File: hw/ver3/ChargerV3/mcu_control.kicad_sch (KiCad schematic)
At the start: 58 parts, among them J6 BMS_Serial, J7 Debug, J8 SWD Debug, J9 USB_B_Micro, Q12 BSS138, Q13 BSS138, Q14 BSS138, Q15 BSS84, Q16 BSS138, Q19 BSS138, Q30 BSS138, SW1 Boot, SW2 Reset, U12 W25Q32JVZP, U18 RP2040, U21 W25Q32JVZP, Y1 12MHz

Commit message: Nearly final charger schematic, updated with RS485 interconnect.
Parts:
- removed C24: 100nF, Capacitor_SMD:C_0603_1608Metric, symbol Device:C
- removed D19: Yellow LED, LED_SMD:LED_0805_2012Metric, symbol Device:LED
- removed J6: BMS_Serial, Connector_PinHeader_2.54mm:PinHeader_1x03_P2.54mm_Vertical, symbol Connector:Conn_01x03_Pin
- removed Q30: BSS138, Package_TO_SOT_SMD:SOT-23, symbol Transistor_FET:BSS138
- removed R115: 510, Resistor_SMD:R_0603_1608Metric, symbol Device:R_US
- removed R5, R97: 10k, Resistor_SMD:R_0603_1608Metric, symbol Device:R_US
- removed R58, R59: 100, Resistor_SMD:R_0603_1608Metric, symbol Device:R_US
- added J5: FanConnector, Connector_Molex:Molex_KK-254_AE-6410-04A_1x04_P2.54mm_Vertical, symbol Connector:Conn_01x04_Pin
- added R55, R56: 100, Resistor_SMD:R_0603_1608Metric, symbol Device:R_US
- added R57: 10k, Resistor_SMD:R_0603_1608Metric, symbol Device:R_US
- added R92: 1k, Resistor_SMD:R_0603_1608Metric, symbol Device:R_US
- J9: footprint Connector_USB:USB_Micro-AB_Molex_47590-0001 -> USB:Amphenol-MicroB; Digikey (none) -> ZX62D-B-5PA8(30); LCSC (none) -> C132350
- SW1, SW2: footprint Button_Switch_SMD:SW_SPST_EVQP2 -> Button_Switch_SMD:SW_Tactile_SPST_NO_Straight_CK_PTS636Sx25SMTRLFS; Digikey P11081SCT-ND -> CKN12321-2-ND; LCSC C2915169 -> C318938
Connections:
- net INTERCONNECT_RTX_EN is gone; now on net LED_STATUS_0: U18.14 (GPIO11)
- net +3.3V: now also R57.2
- net GND: now also J5.1 (Pin_1)
- net LED_STATUS_0: no longer U18.29 (GPIO18)
- net PWM_FAN_CTL: now also R56.2
- net PWM_FAN_SENSE: now also R55.1, R57.1
- net QSPI_SS: now also R92.2
- net RUN: no longer SW2.2, U18.26 (RUN)
- net UART0_RX: now also R74.2
- net UART0_TX: now also R60.2
- net at R109.2: now also D22.2 (A)
- net at Q19.3 (D): now also D22.1 (K)
- net at SW1.2: now also R92.1
- net ISENSE_OUTPUT: now reaches U18.38 (GPIO26_ADC0)
- net ISENSE_INPUT: now reaches U18.41 (GPIO29_ADC3)
- net LED_STATUS_1 renamed RS485_ACTIVITY_LED
- net UART1_RX renamed RS485_DATA_IN
- net UART1_TX renamed RS485_DATA_OUT
- new net: J5.4 (Pin_4), R56.1
- new net: J5.3 (Pin_3), R55.2
- new net: SW2.2, U18.26 (RUN)
- new net +12V: J5.2 (Pin_2)
- new net RS485_DATA_DIR: U18.29 (GPIO18)
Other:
- note added: "Board IO"
- note added: "Discrete Control"
- note added: "External Memory"
- note added: "Provides software control/inspection of: - LTC7871 operating state - ADC Sensor Data - System logging and config - External network interface over RS485"
- note added: "RP2040 MCU"
- note removed: "1. Add CAN bus ports. Likely two? Alternatively RS485 or something. 2. Ensure charger board connector is large enough to handle future expansion 3. Ensure charger IO are 5v tolerant (bidirectional) 4. Add RJ45 connectors to talk to multiple balancers 5. Add RJ45 connectors to talk to multiple inverters 6. Am I building a DCU + HID? 7. Do I need to provision for a WiFi Connection? Maybe an ESP32 i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"
- moved on the sheet: C100, C108, C111, C114, C115, C118, C119, C121, C123, C124, C125, C126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

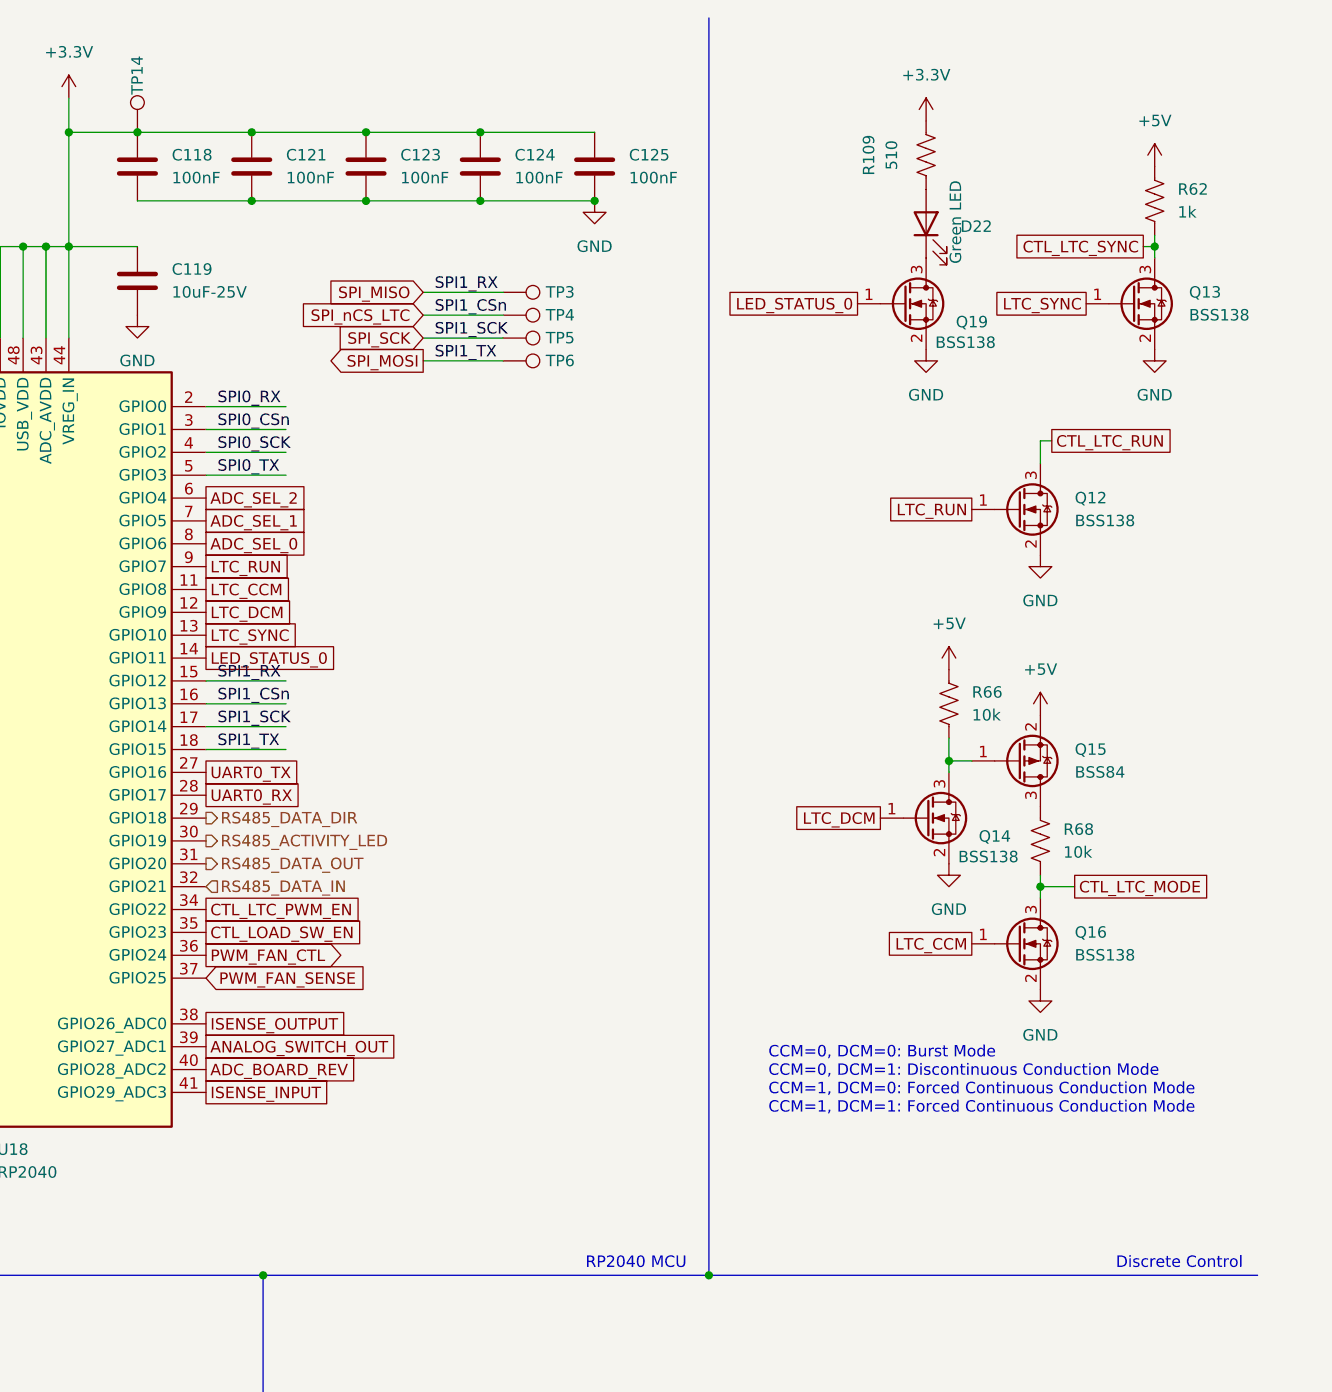
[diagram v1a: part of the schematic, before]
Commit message: Sync board changes from before work started
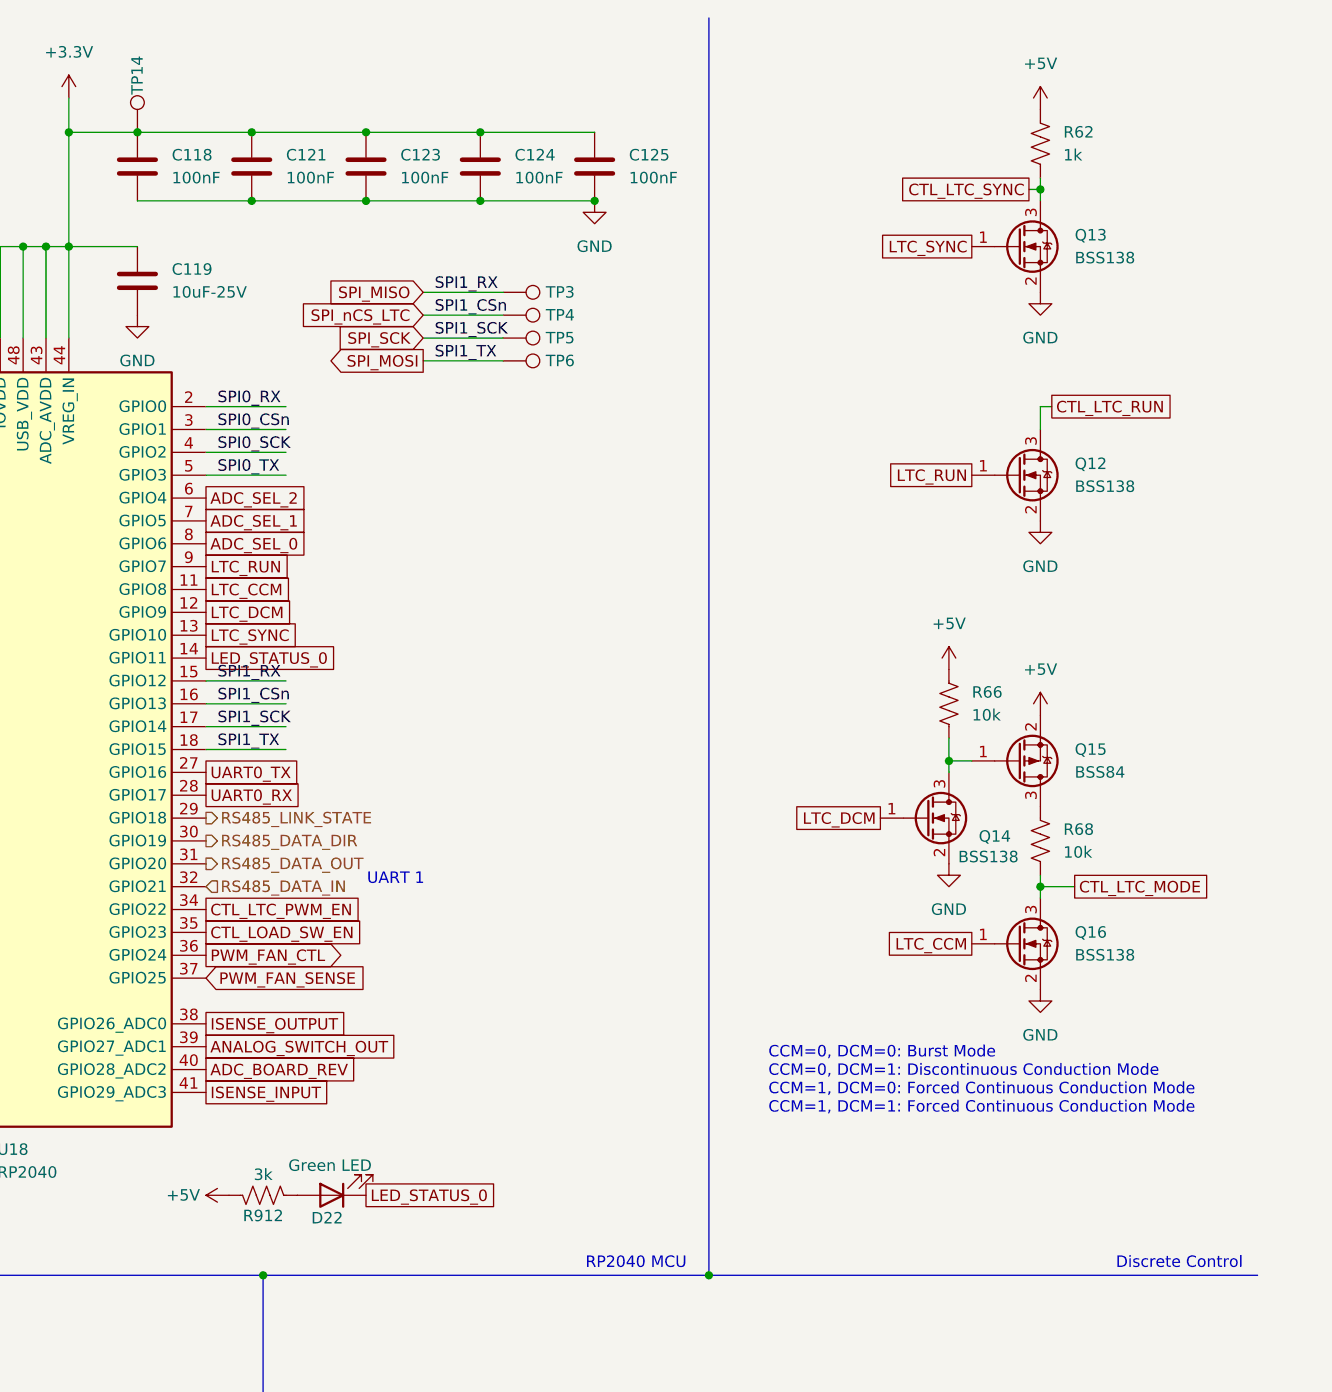
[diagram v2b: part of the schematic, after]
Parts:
- removed Q19: BSS138, Package_TO_SOT_SMD:SOT-23, symbol Transistor_FET:BSS138
- removed R109: 510, Resistor_SMD:R_0603_1608Metric, symbol Device:R_US
- added R912: 3k, Resistor_SMD:R_0603_1608Metric, symbol Device:R_US
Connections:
- net RS485_ACTIVITY_LED is gone; now on net RS485_DATA_DIR: U18.30 (GPIO19)
- net +5V: now also R912.2
- net LED_STATUS_0: now also D22.1 (K)
- net RS485_DATA_DIR: no longer U18.29 (GPIO18)
- net at D22.2 (A): now also R912.1
- new net RS485_LINK_STATE: U18.29 (GPIO18)
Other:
- note added: "UART 1"
- moved on the sheet: D22, Q12, Q13, R62
